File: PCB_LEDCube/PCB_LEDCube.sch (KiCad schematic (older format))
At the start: 72 parts, among them J1 Source, J2 Batt, Q1 2N2219, Q10 2N2219, Q2 2N2219, Q3 2N2219, Q4 2N2219, Q5 2N2219, Q6 2N2219, Q7 2N2219, Q8 2N2219, Q9 2N2219, U1 L7805, U2 MCP73931, U3 WemosESP32, U4 74HC595, U5 74HC595

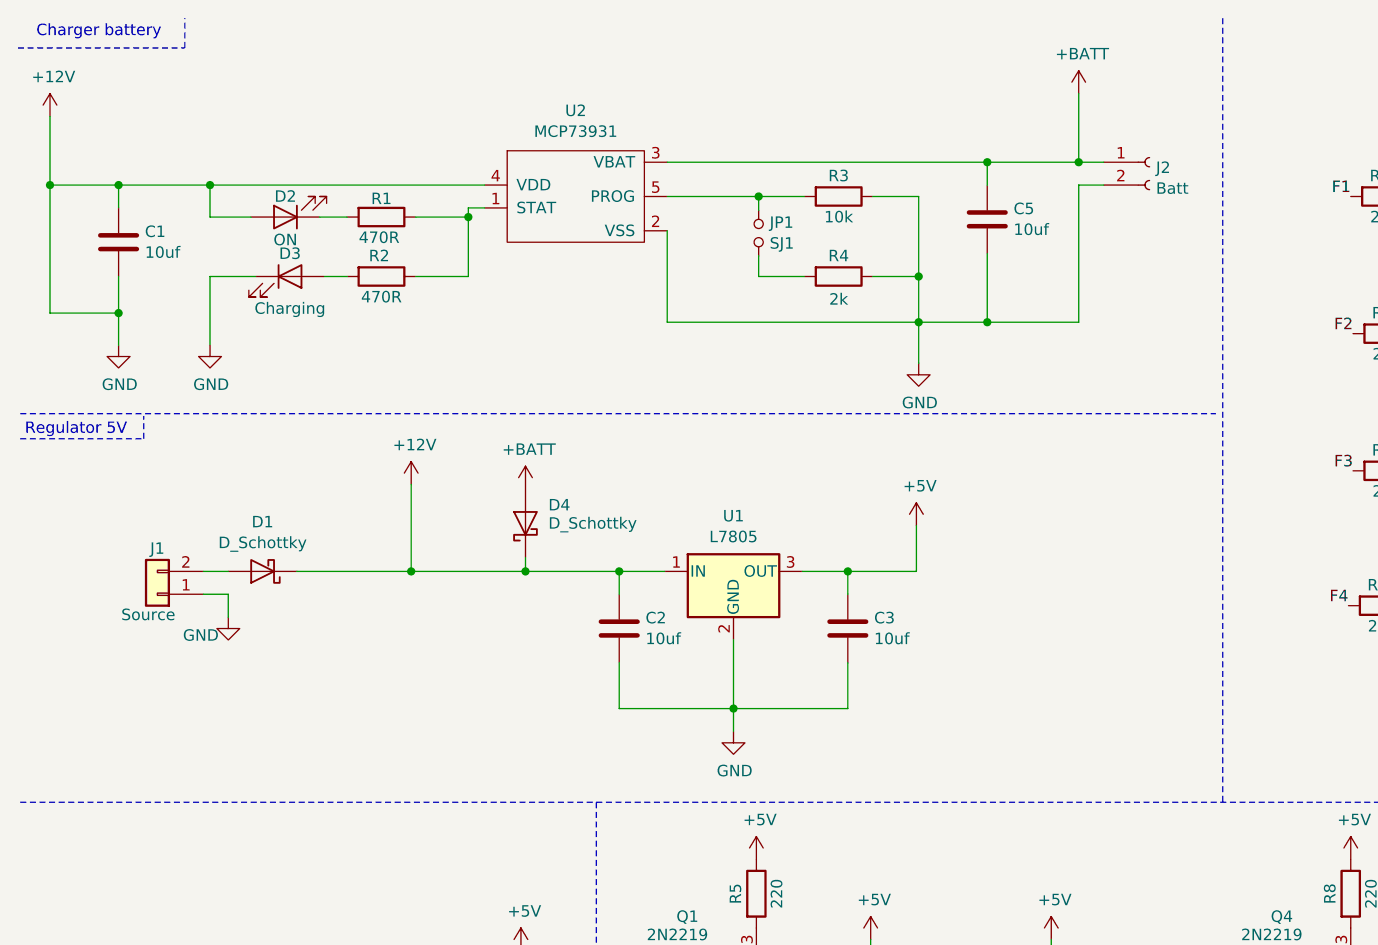
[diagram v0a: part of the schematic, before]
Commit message: PCB TH hand
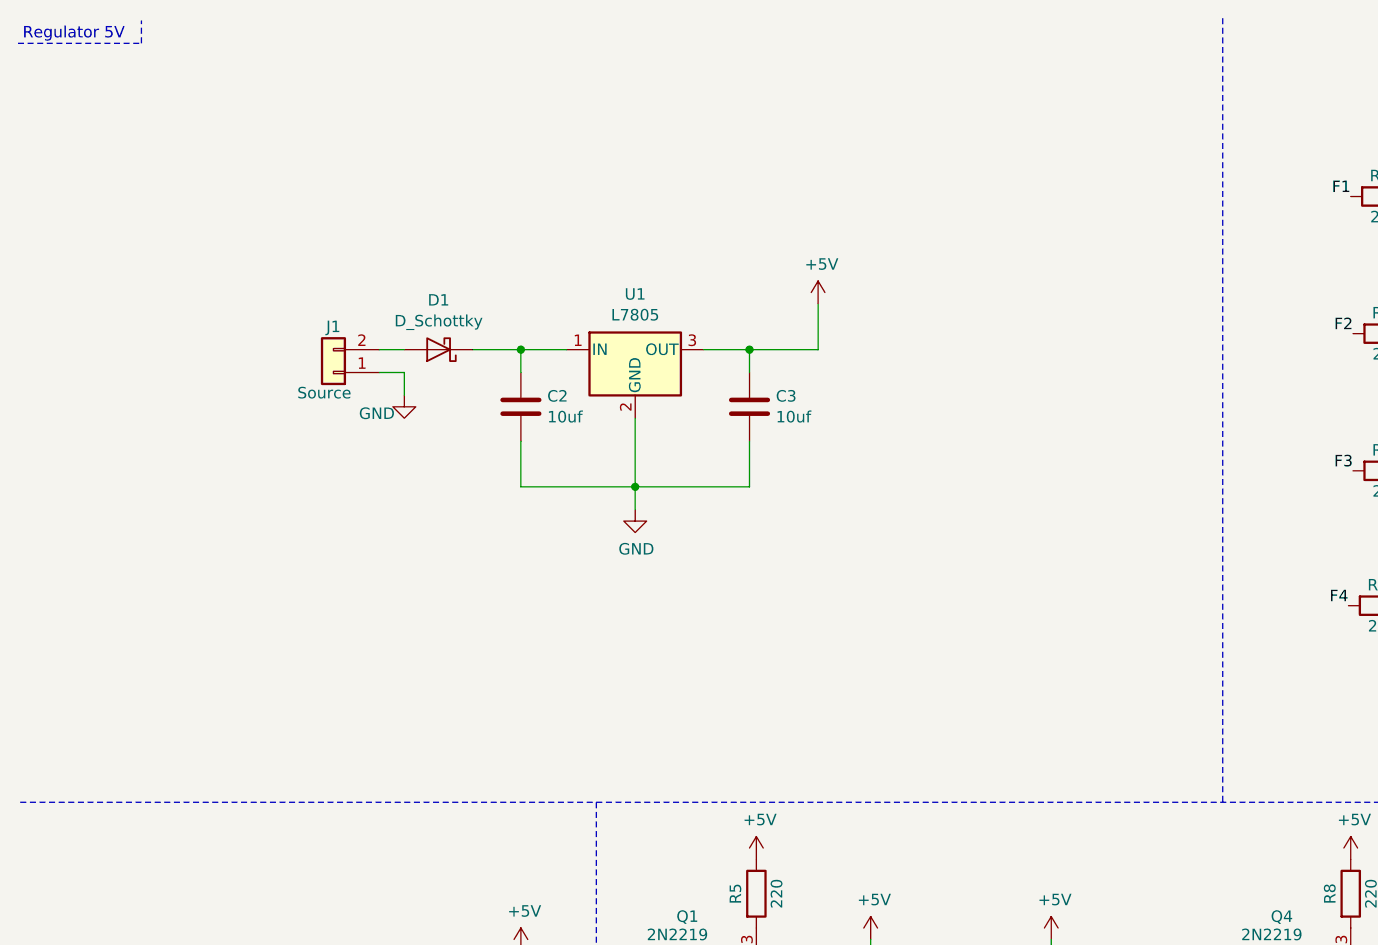
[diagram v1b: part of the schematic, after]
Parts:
- removed C1, C5: 10uf, Capacitor_SMD:C_1206_3216Metric_Pad1.42x1.75mm_HandSolder, symbol Device:C
- removed D2: ON, LED_SMD:LED_1206_3216Metric_Pad1.42x1.75mm_HandSolder, symbol Device:LED
- removed D3: Charging, LED_SMD:LED_1206_3216Metric_Pad1.42x1.75mm_HandSolder, symbol Device:LED
- removed D4: D_Schottky, Diode_THT:D_A-405_P7.62mm_Horizontal, symbol Device:D_Schottky
- removed J2: Batt, Connector_PinHeader_2.54mm:PinHeader_1x02_P2.54mm_Vertical, symbol Connector:Conn_01x02_Female
- removed JP1: SJ1, Jumper:SolderJumper-2_P1.3mm_Open_RoundedPad1.0x1.5mm, symbol Device:Jumper_NO_Small
- removed R1, R2: 470R, Resistor_SMD:R_1206_3216Metric_Pad1.42x1.75mm_HandSolder, symbol Device:R
- removed R3: 10k, Resistor_SMD:R_1206_3216Metric_Pad1.42x1.75mm_HandSolder, symbol Device:R
- removed R4: 2k, Resistor_SMD:R_1206_3216Metric_Pad1.42x1.75mm_HandSolder, symbol Device:R
- removed U2: MCP73931, Package_TO_SOT_SMD:SOT-23-5, symbol PCB_LEDCube-rescue:MCP73931-Regulator
- C2, C3: footprint Capacitor_SMD:C_1206_3216Metric_Pad1.42x1.75mm_HandSolder -> Capacitor_THT:C_Disc_D5.0mm_W2.5mm_P5.00mm
- R10, R11, R12, R13, R14, R15, R16, R17, R18, R19, R20, R21, R22, R23, R24, R25, R26, R27, R28, R29, R30, R5, R6, R7, R8, R9: footprint Resistor_SMD:R_1206_3216Metric_Pad1.42x1.75mm_HandSolder -> Resistor_THT:R_Axial_DIN0207_L6.3mm_D2.5mm_P7.62mm_Horizontal
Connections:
- net +12V renamed GND
- net GND: no longer C2.1, D1.1 (K), U1.1 (IN)
- new net: C2.1, D1.1 (K), U1.1 (IN)
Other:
- note removed: "Charger battery"
- moved on the sheet: C2, C3, D1, J1, U1
